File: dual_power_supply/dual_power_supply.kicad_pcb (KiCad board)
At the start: 2 copper layers, 45.7 x 24.4 mm, 15 parts, among them J1 Screw_Terminal_01x02, J2 Screw_Terminal_01x02, J3 Screw_Terminal_01x02, SW1 SW_DIP_x01, SW2 SW_DIP_x01, U1 LD1117S33TR_SOT223, U2 LD1117S50TR_SOT223

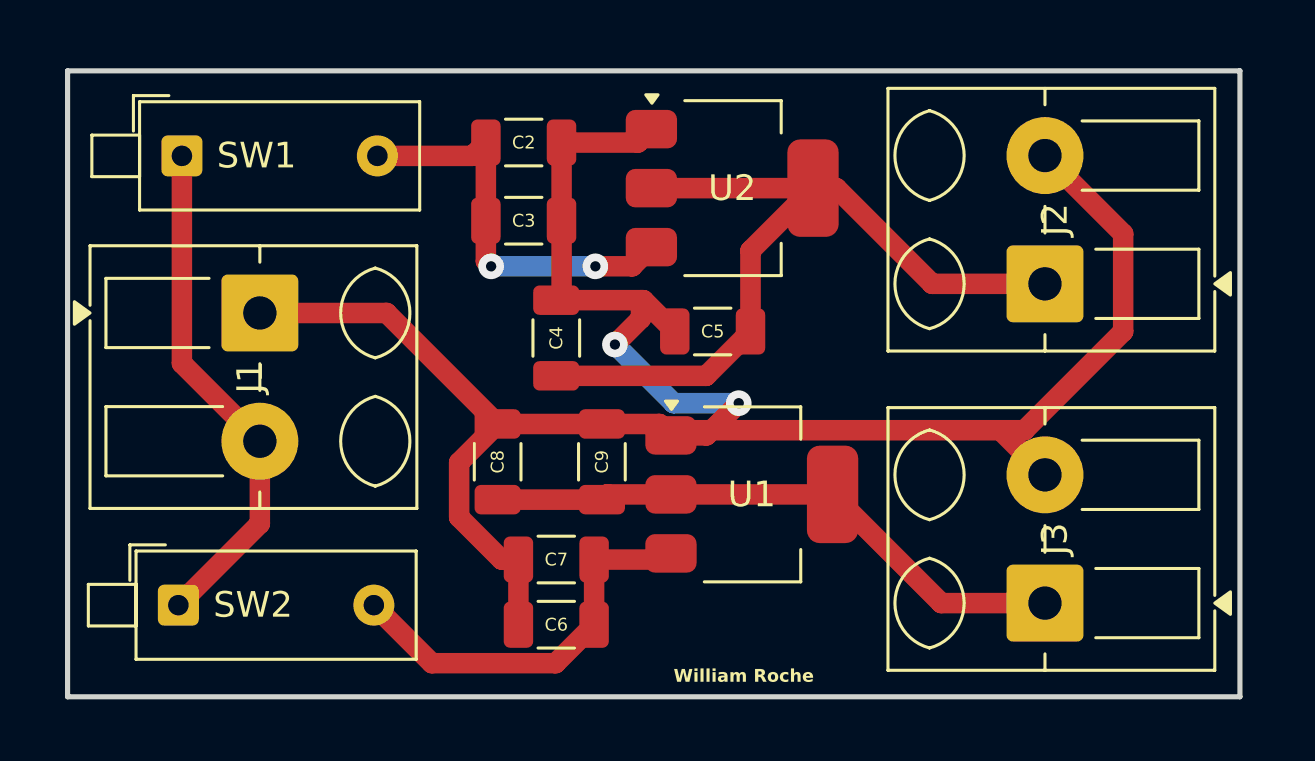
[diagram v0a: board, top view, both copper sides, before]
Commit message: Add files via upload
updated
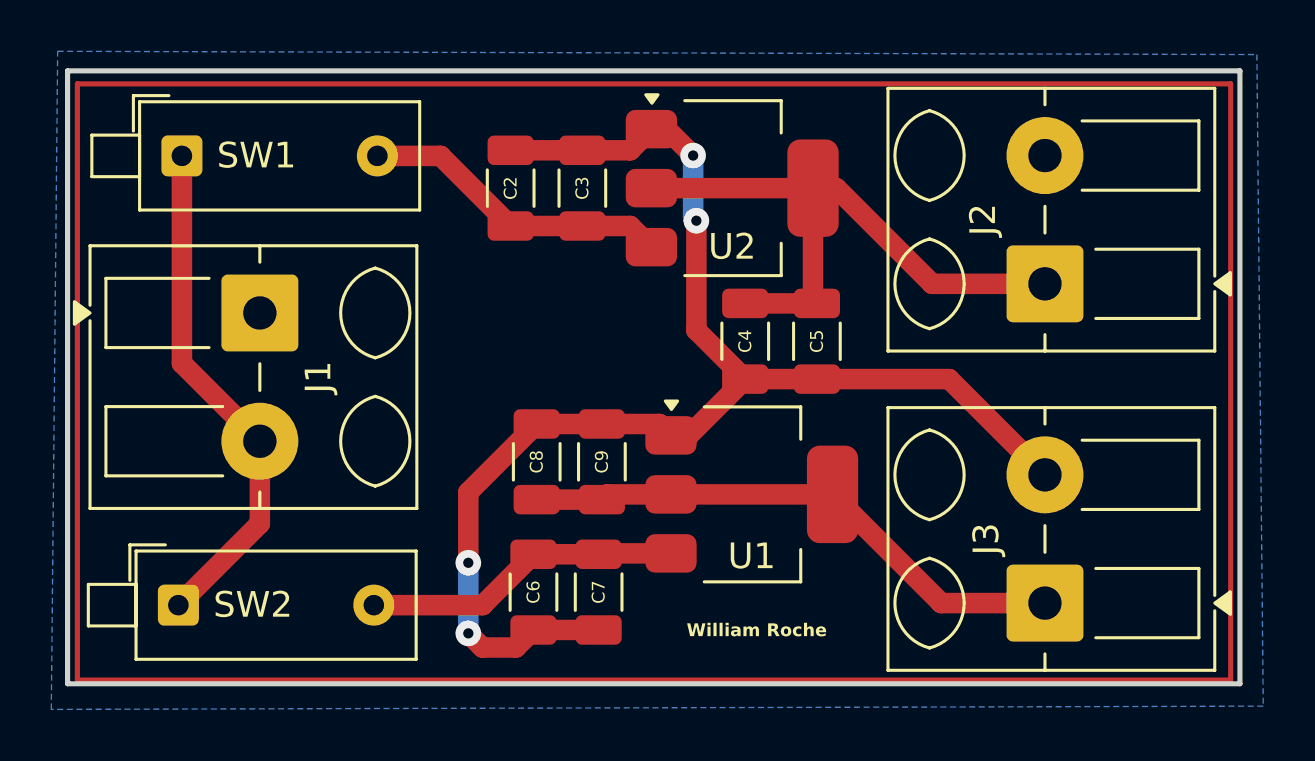
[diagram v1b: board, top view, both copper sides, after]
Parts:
- moved C4 7.37 mm to (130.8, 90.6), turned to -90 degrees
- moved C5 4.08 mm to (133.6, 90.6), turned to -90 degrees
- moved C3 2.62 mm to (124.5, 84.6), turned to 90 degrees
- moved C7 2.08 mm to (125.1, 100.3), turned to -90 degrees
- moved C2 1.85 mm to (121.7, 84.6), turned to 90 degrees
- moved C6 1.55 mm to (122.6, 100.3), turned to -90 degrees
- moved C8 1.52 mm to (122.7, 95.2)
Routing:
- net GND: track 83.8 -> 55.0 mm, vias 2 -> 4
- net Net-(J2-Pin_1): track 31.8 -> 24.2 mm
- net Net-(U2-VI): track 15.9 -> 12.2 mm, vias 2 -> 0
- net Net-(U1-VI): track 15.8 -> 12.8 mm
- net Net-(J3-Pin_1): track 23.2 -> 21.7 mm
- added copper zone on B.Cu, net GND
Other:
- board size 45.7 x 24.4 mm -> 45.7 x 23.9 mm
